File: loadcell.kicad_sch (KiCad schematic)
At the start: 11 parts, among them J31 DSUB_15pin/VGA Veritical Fema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, U33 INA126

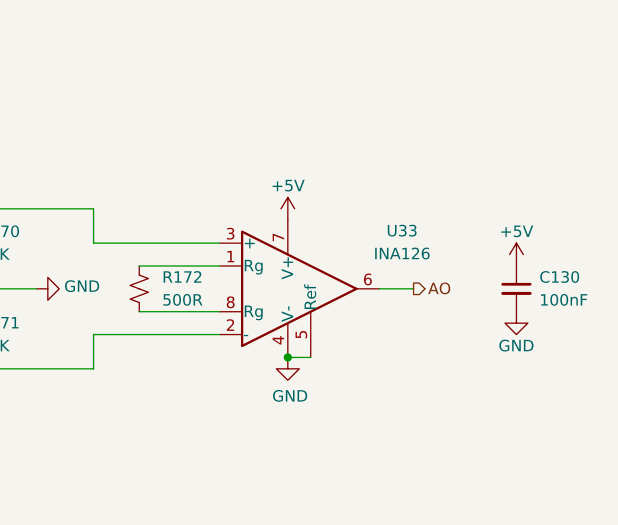
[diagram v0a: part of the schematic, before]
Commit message: GSE v2.1 done, just waiting on prop rn to finalize their sensor list
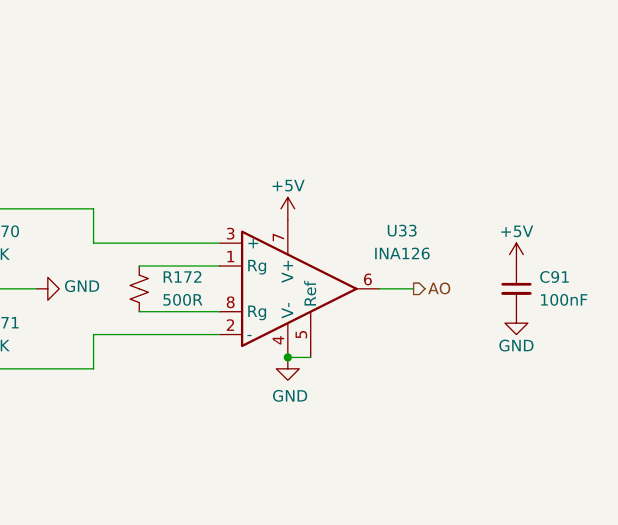
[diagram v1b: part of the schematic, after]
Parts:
- removed U33: INA126, Package_SO:SOIC-8_3.9x4.9mm_P1.27mm, symbol Amplifier_Instrumentation:INA128
- added U33: INA126, 0UCIRP-KiCAD-Lib:Instrumentation_Amplifiers INA126, symbol 0UCIRP-KiCAD-Lib:Instrumentation_Amplifiers INA126
- renumbered C130 to C91
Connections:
- net +5V: now also U33.7 (V+)
- net AO: now also U33.6
- net GND: now also U33.4 (V-), U33.5 (Ref)
- net at R172.2: now also U33.1 (Rg)
- net at C88.2, C90.1, R169.2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: now also U33.2 (-)
- net at C88.1, C89.2, R168.1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: now also U33.3 (+)
- net at R172.1: now also U33.8 (Rg)
